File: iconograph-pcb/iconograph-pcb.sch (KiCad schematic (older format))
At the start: 38 parts, among them J1 Conn_01x02, J10 105162-0001, J11 Conn_01x04, J12 Conn_01x04, J13 Conn_01x04, J2 Conn_01x03, J3 Anderson_two_redblack_src, J4 Conn_01x02, J5 Conn_01x03, J6 Conn_01x02, J7 Conn_01x05, J8 Conn_01x02, J9 Conn_01x02, SW1 SW_DIP_x03, SW2 SW_DIP_x03, SW3 SW_DIP_x03, SW4 SW_SPST, SW5 SW_SPST, SW6 SW_SPST, SW7 SW_SPST, U1 mini_esp32, U2 ULN2003

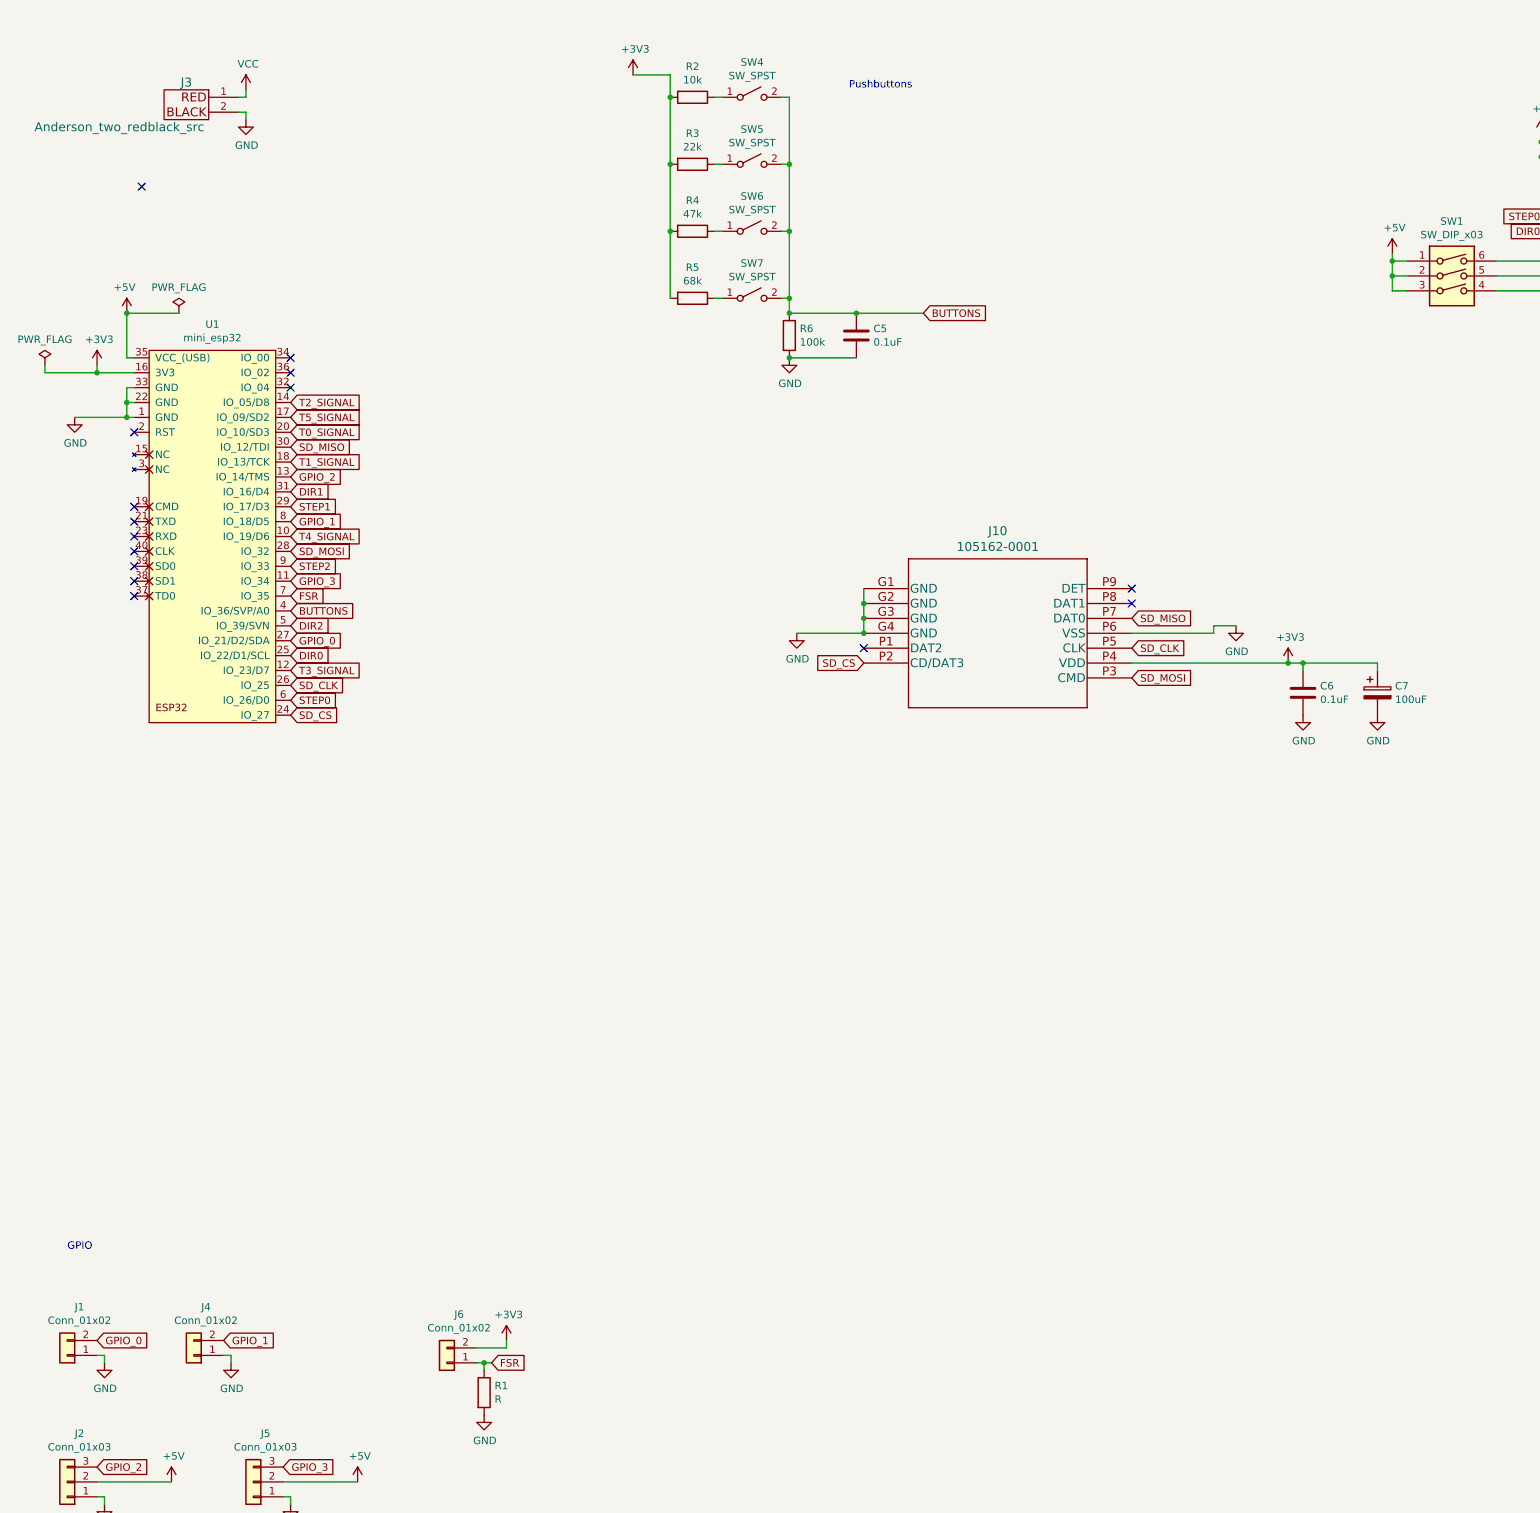
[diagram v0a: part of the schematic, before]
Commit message: PCB v1.0
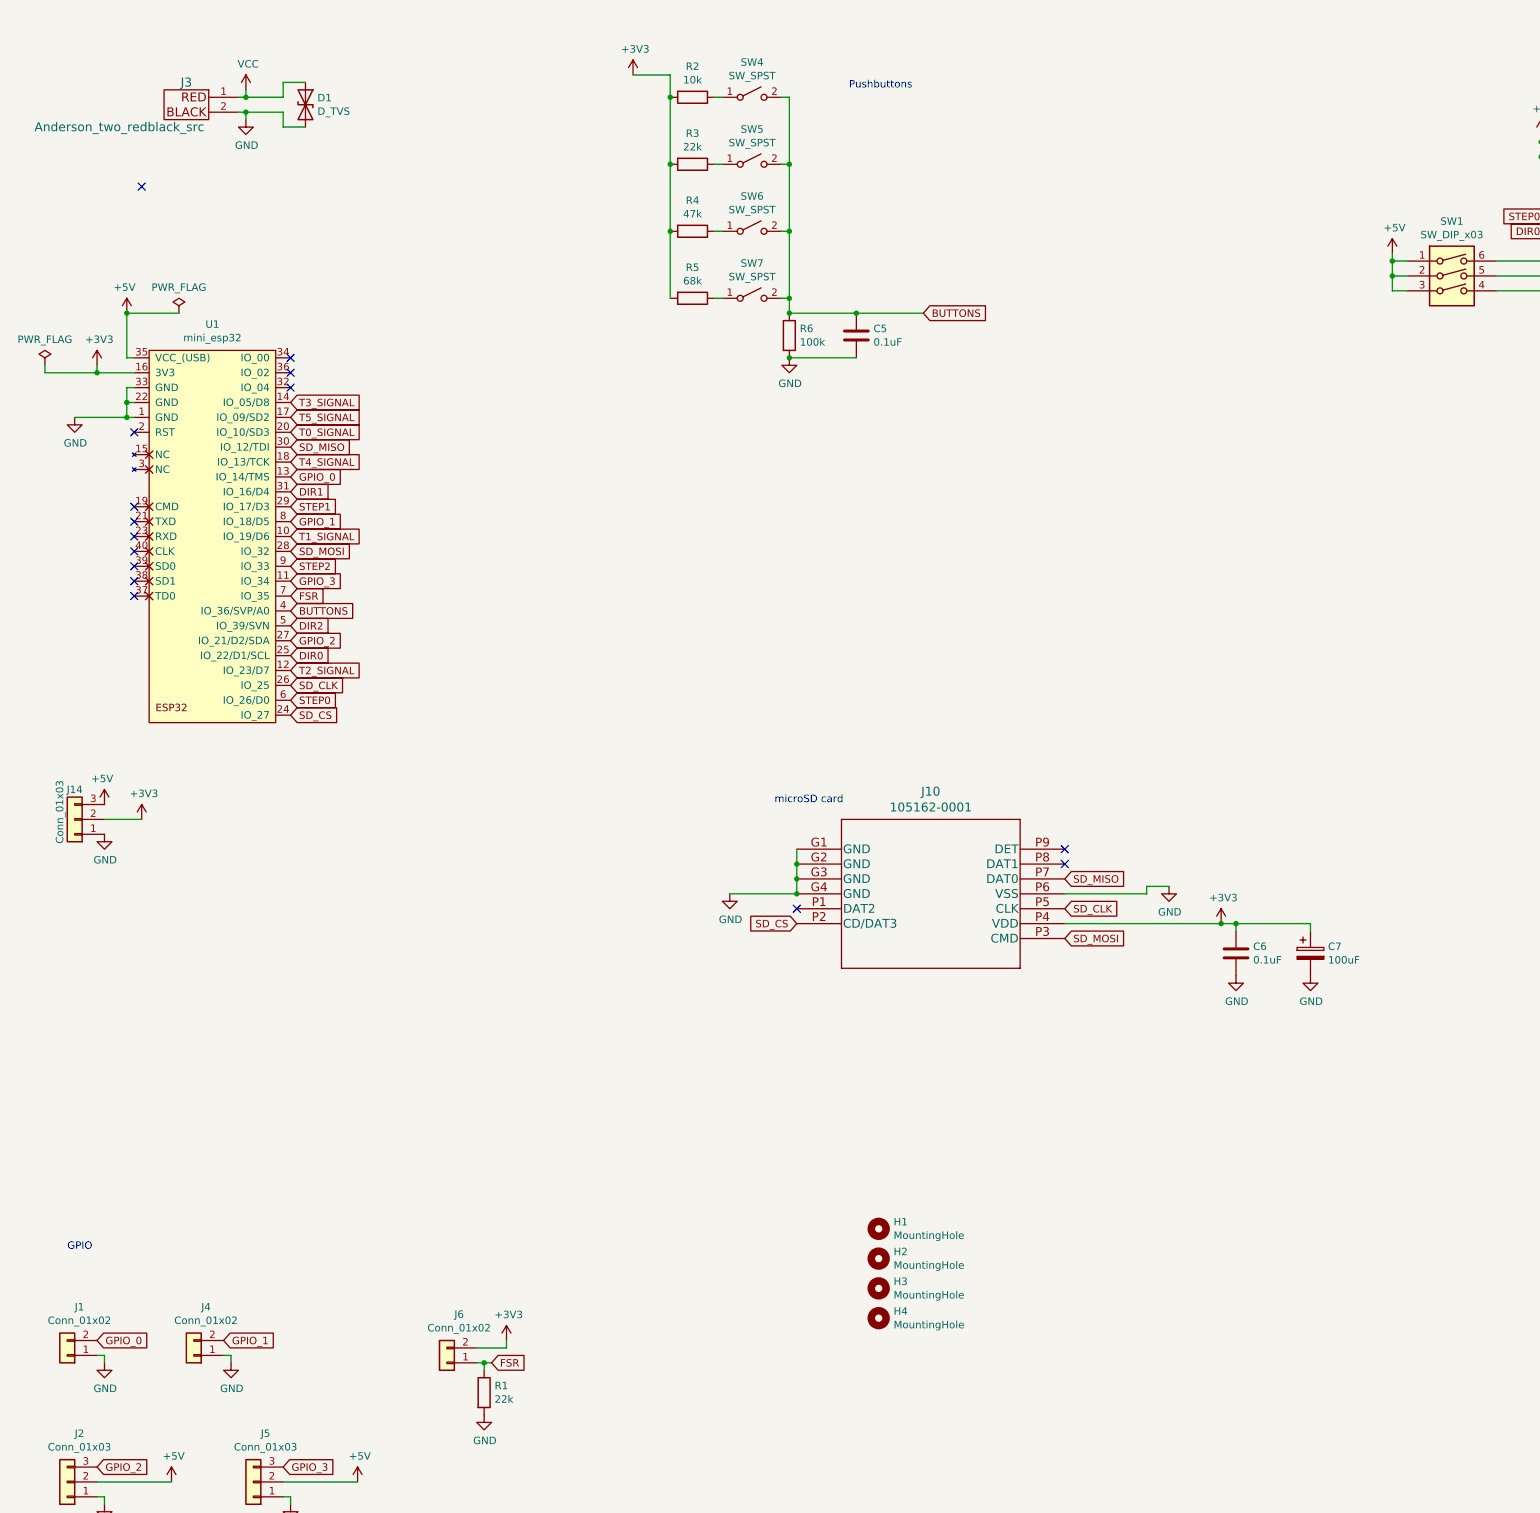
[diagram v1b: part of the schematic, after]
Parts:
- added D1: D_TVS, Diode_THT:D_DO-15_P10.16mm_Horizontal, symbol Device:D_TVS
- added H1, H2, H3, H4: MountingHole, MountingHole:MountingHole_3.2mm_M3, symbol Mechanical:MountingHole
- added J14: Conn_01x03, homebrew:Wurth_ScrewTerminal_1x03_P5.00mm_691137710003, symbol Connector_Generic:Conn_01x03
- C1, C2, C3, C4, C7: footprint (none) -> Capacitor_THT:CP_Radial_D8.0mm_P3.50mm
- C5, C6: footprint (none) -> Capacitor_THT:C_Disc_D5.1mm_W3.2mm_P5.00mm
- J1, J4, J6, J8, J9: footprint (none) -> homebrew:Wurth_ScrewTerminal_1x02_P5.00mm_691137710002
- J11, J12, J13: footprint (none) -> Connector_PinHeader_2.54mm:PinHeader_1x04_P2.54mm_Vertical
- J2, J5: footprint (none) -> homebrew:Wurth_ScrewTerminal_1x03_P5.00mm_691137710003
- J3: footprint (none) -> homebrew:Anderson_1336G1_right_angle_bottom_two
- J7: footprint (none) -> Connector_PinHeader_2.54mm:PinHeader_1x05_P2.54mm_Vertical
- R1: value R -> 22k; footprint (none) -> Resistor_THT:R_Axial_DIN0207_L6.3mm_D2.5mm_P7.62mm_Horizontal
- R2, R3, R4, R5, R6: footprint (none) -> Resistor_THT:R_Axial_DIN0207_L6.3mm_D2.5mm_P7.62mm_Horizontal
- SW1, SW2, SW3: footprint (none) -> Button_Switch_THT:SW_DIP_SPSTx03_Slide_9.78x9.8mm_W7.62mm_P2.54mm
- SW4, SW5, SW6, SW7: footprint (none) -> snapeda:SW_1825910-6-4
- U1: footprint (none) -> snapeda:ESP32_mini
- U2: footprint (none) -> Package_DIP:DIP-16_W7.62mm
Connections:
- net +3V3: now also J14.2 (Pin_2)
- net +5V: now also J14.3 (Pin_3)
- net GND: now also D1.2 (A2), J14.1 (Pin_1)
- net GPIO_0: now also U1.13 (IO_14/TMS); no longer U1.27 (IO_21/D2/SDA)
- net GPIO_2: now also U1.27 (IO_21/D2/SDA); no longer U1.13 (IO_14/TMS)
- net T1_SIGNAL: now also U1.10 (IO_19/D6); no longer U1.18 (IO_13/TCK)
- net T2_SIGNAL: now also U1.12 (IO_23/D7); no longer U1.14 (IO_05/D8)
- net T3_SIGNAL: now also U1.14 (IO_05/D8); no longer U1.12 (IO_23/D7)
- net T4_SIGNAL: now also U1.18 (IO_13/TCK); no longer U1.10 (IO_19/D6)
- net VCC: now also D1.1 (A1)
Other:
- note added: "microSD card"
- moved on the sheet: C6, C7, J10
